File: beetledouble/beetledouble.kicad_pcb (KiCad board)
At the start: 4 copper layers, 31 x 59 mm, 49 parts, among them J1 power in, J2 rxin, J4 motor_out, J5 motor_out, J6 prog connector, Q1 IPG20N04S4-12, Q2 IPG20N04S4-12, Q3 IPG20N04S4-12, Q4 IPG20N04S4-12, U1 78L12G-AB3-R, U2 DD4012SB, U3 ATtiny1614-SS, U4 NCP81155MNTXG, U5 NCP81155MNTXG, U6 NCP81155MNTXG, U7 NCP81155MNTXG

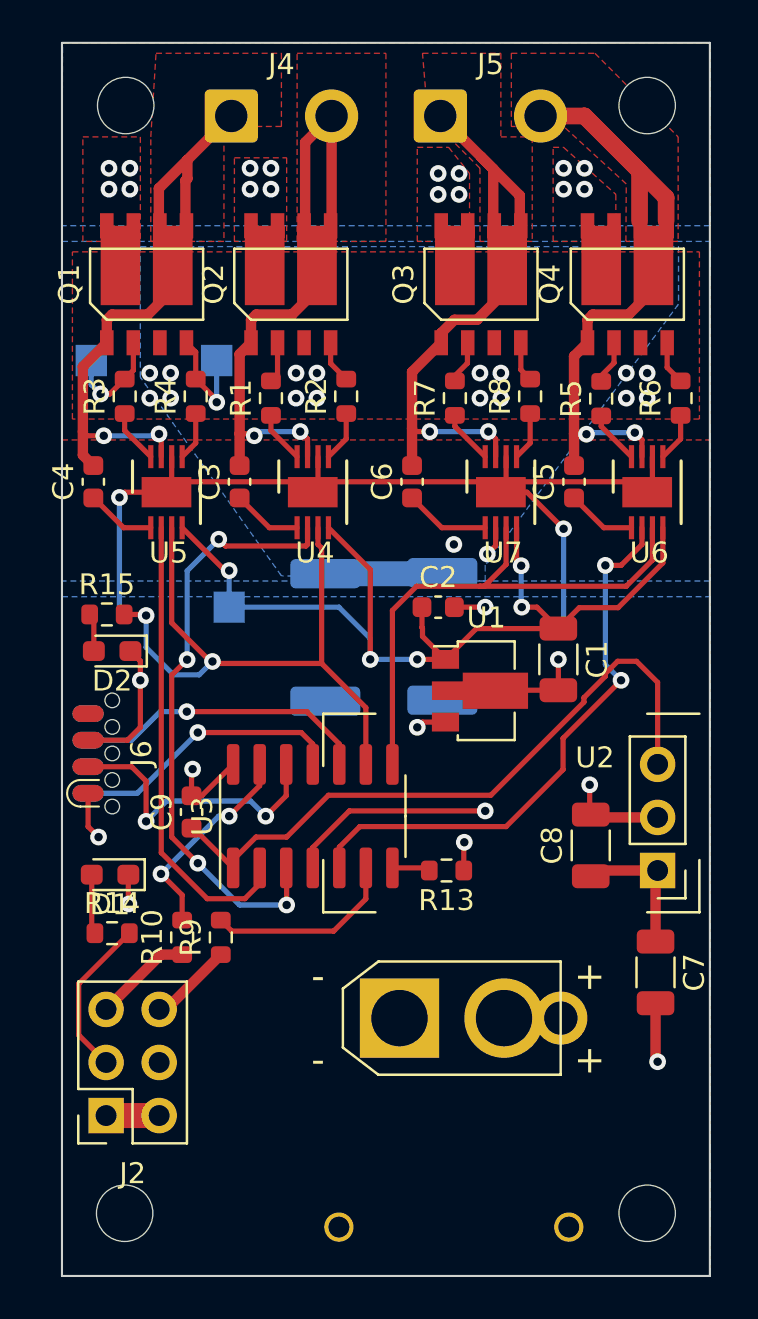
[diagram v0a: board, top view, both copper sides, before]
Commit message: Beetledouble: tweaks
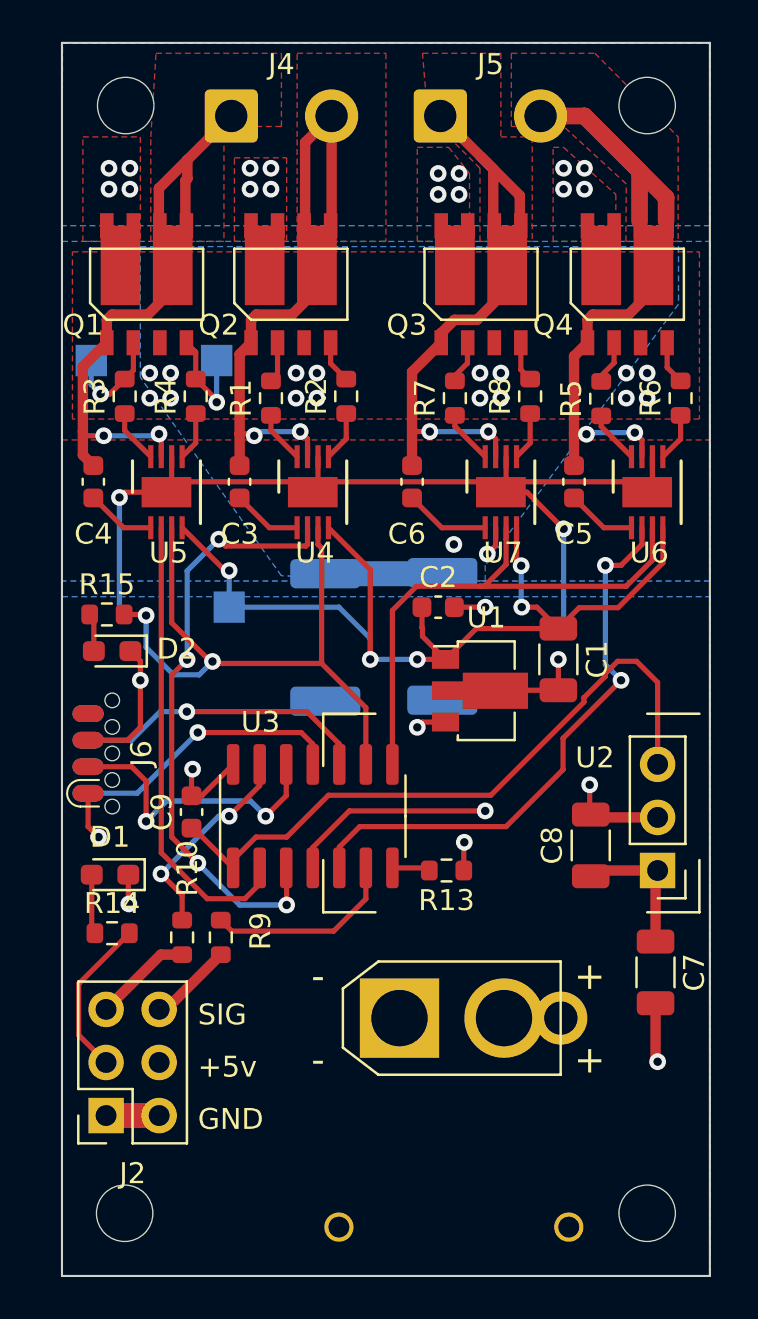
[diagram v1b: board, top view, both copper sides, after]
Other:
- board text added: "+5v"
- board text added: "GND"
- board text added: "SIG"
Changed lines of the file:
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@@
     (property "Sheetname" "driver1")
     (attr smd)
-    (fp_text reference "C4" (at 0 -1.43 90) (layer "F.SilkS")
+    (fp_text reference "C4" (at -2.5 0 180) (layer "F.SilkS")
       (effects (font (size 1 1) (thickness 0.15)))
     )
@@
     (property "Sheetname" "driver2")
     (attr through_hole)
-    (fp_text reference "Q3" (at -3.705 0 90) (layer "F.SilkS")
+    (fp_text reference "Q3" (at -3.55 1.95 180) (layer "F.SilkS")
       (effects (font (size 1 1) (thickness 0.15)))
     )
@@
     (property "Sheetname" "driver2")
     (attr smd)
-    (fp_text reference "C6" (at 0 -1.43 90) (layer "F.SilkS")
+    (fp_text reference "C6" (at -2.5 -0.25 180) (layer "F.SilkS")
       (effects (font (size 1 1) (thickness 0.15)))
     )
@@
     (property "Sheetname" "driver1")
     (attr through_hole)
-    (fp_text reference "Q1" (at -3.705 0 90) (layer "F.SilkS")
+    (fp_text reference "Q1" (at -3.05 1.95 180) (layer "F.SilkS")
       (effects (font (size 1 1) (thickness 0.15)))
     )
@@
     (property "Sheetname" "")
     (attr smd)
-    (fp_text reference "R10" (at 0 -1.43 90) (layer "F.SilkS")
+    (fp_text reference "R10" (at 3.3 0.25 90) (layer "F.SilkS")
       (effects (font (size 1 1) (thickness 0.15)))
     )
@@
     (property "Sheetname" "")
     (attr smd)
-    (fp_text reference "D1" (at 0 -1.43) (layer "F.SilkS")
+    (fp_text reference "D1" (at 0 1.8) (layer "F.SilkS")
       (effects (font (size 1 1) (thickness 0.15)))
     )
@@
     (property "Sheetname" "driver1")
     (attr through_hole)
-    (fp_text reference "Q2" (at -3.705 0 90) (layer "F.SilkS")
+    (fp_text reference "Q2" (at -3.45 1.95 180) (layer "F.SilkS")
       (effects (font (size 1 1) (thickness 0.15)))
     )
@@
     (property "Sheetname" "driver2")
     (attr through_hole)
-    (fp_text reference "Q4" (at -3.705 0 90) (layer "F.SilkS")
+    (fp_text reference "Q4" (at -3.55 1.95 180) (layer "F.SilkS")
       (effects (font (size 1 1) (thickness 0.15)))
     )
@@
     (property "Sheetname" "")
     (attr smd)
-    (fp_text reference "D2" (at 0 -1.43) (layer "F.SilkS")
+    (fp_text reference "D2" (at -3.1 0.1) (layer "F.SilkS")
       (effects (font (size 1 1) (thickness 0.15)))
     )
@@
     (property "Sheetname" "driver1")
     (attr smd)
-    (fp_text reference "C3" (at 0 -1.43 90) (layer "F.SilkS")
+    (fp_text reference "C3" (at -2.5 0 180) (layer "F.SilkS")
       (effects (font (size 1 1) (thickness 0.15)))
     )
@@
     (property "Sheetname" "driver2")
     (attr smd)
-    (fp_text reference "C5" (at 0 -1.43 90) (layer "F.SilkS")
+    (fp_text reference "C5" (at -2.5 0 180) (layer "F.SilkS")
       (effects (font (size 1 1) (thickness 0.15)))
     )
@@
     (property "Sheetname" "")
     (attr smd)
-    (fp_text reference "U3" (at 0 -5.28 90) (layer "F.SilkS")
+    (fp_text reference "U3" (at 4.5 -2.5 180) (layer "F.SilkS")
       (effects (font (size 1 1) (thickness 0.15)))
     )
@@
     (property "Sheetname" "")
     (attr smd)
-    (fp_text reference "R9" (at 0 -1.43 90) (layer "F.SilkS")
+    (fp_text reference "R9" (at 0.3 1.9 90) (layer "F.SilkS")
       (effects (font (size 1 1) (thickness 0.15)))
     )
@@
   )
   (gr_rect (start 106 72) (end 137 131) (layer "Edge.Cuts") (width 0.1) (fill none))
+  (gr_text "+5v" (at 112.5 121) (layer "F.SilkS")
+    (effects (font (size 1 1) (thickness 0.15)) (justify left))
+  )
+  (gr_text "SIG" (at 112.5 118.5) (layer "F.SilkS")
+    (effects (font (size 1 1) (thickness 0.15)) (justify left))
+  )
+  (gr_text "GND" (at 112.5 123.5) (layer "F.SilkS")
+    (effects (font (size 1 1) (thickness 0.15)) (justify left))
+  )
   (dimension (type aligned) (layer "Dwgs.User")
     (pts (xy 106 131) (xy 137 131))
